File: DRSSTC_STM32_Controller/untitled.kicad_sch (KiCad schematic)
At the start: 46 parts, among them J4 Screw_Terminal_01x02, U3 LF15_TO252, U4 TPS54560BDDA, U7 LV2842XLVDDCR

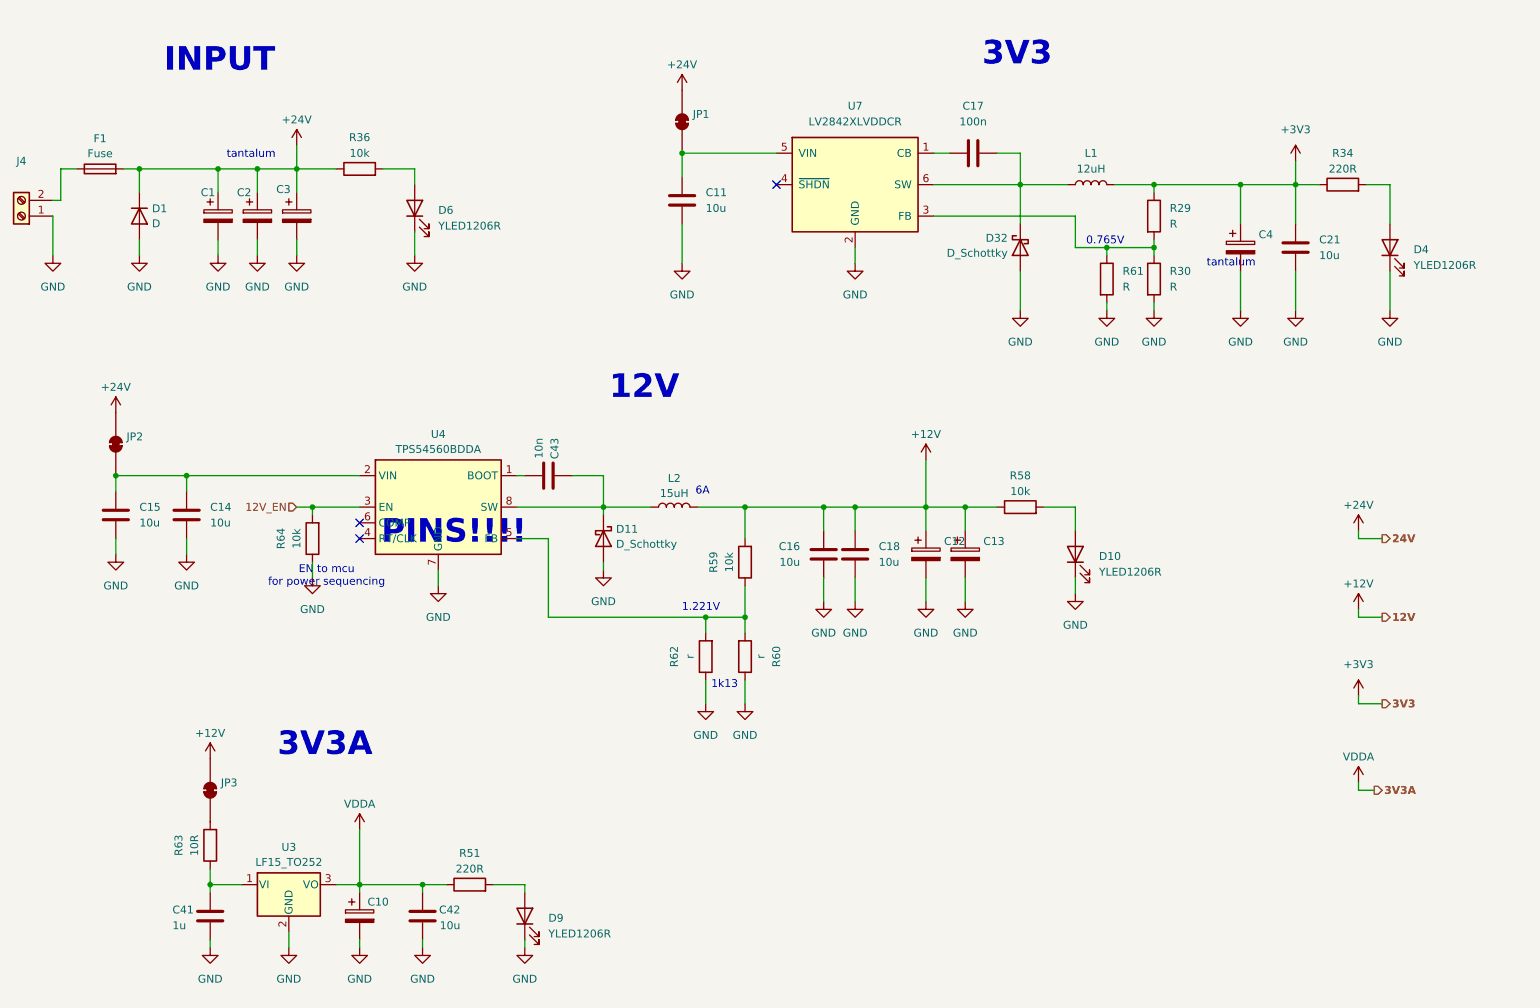
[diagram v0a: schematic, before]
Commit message: update conroller schematics
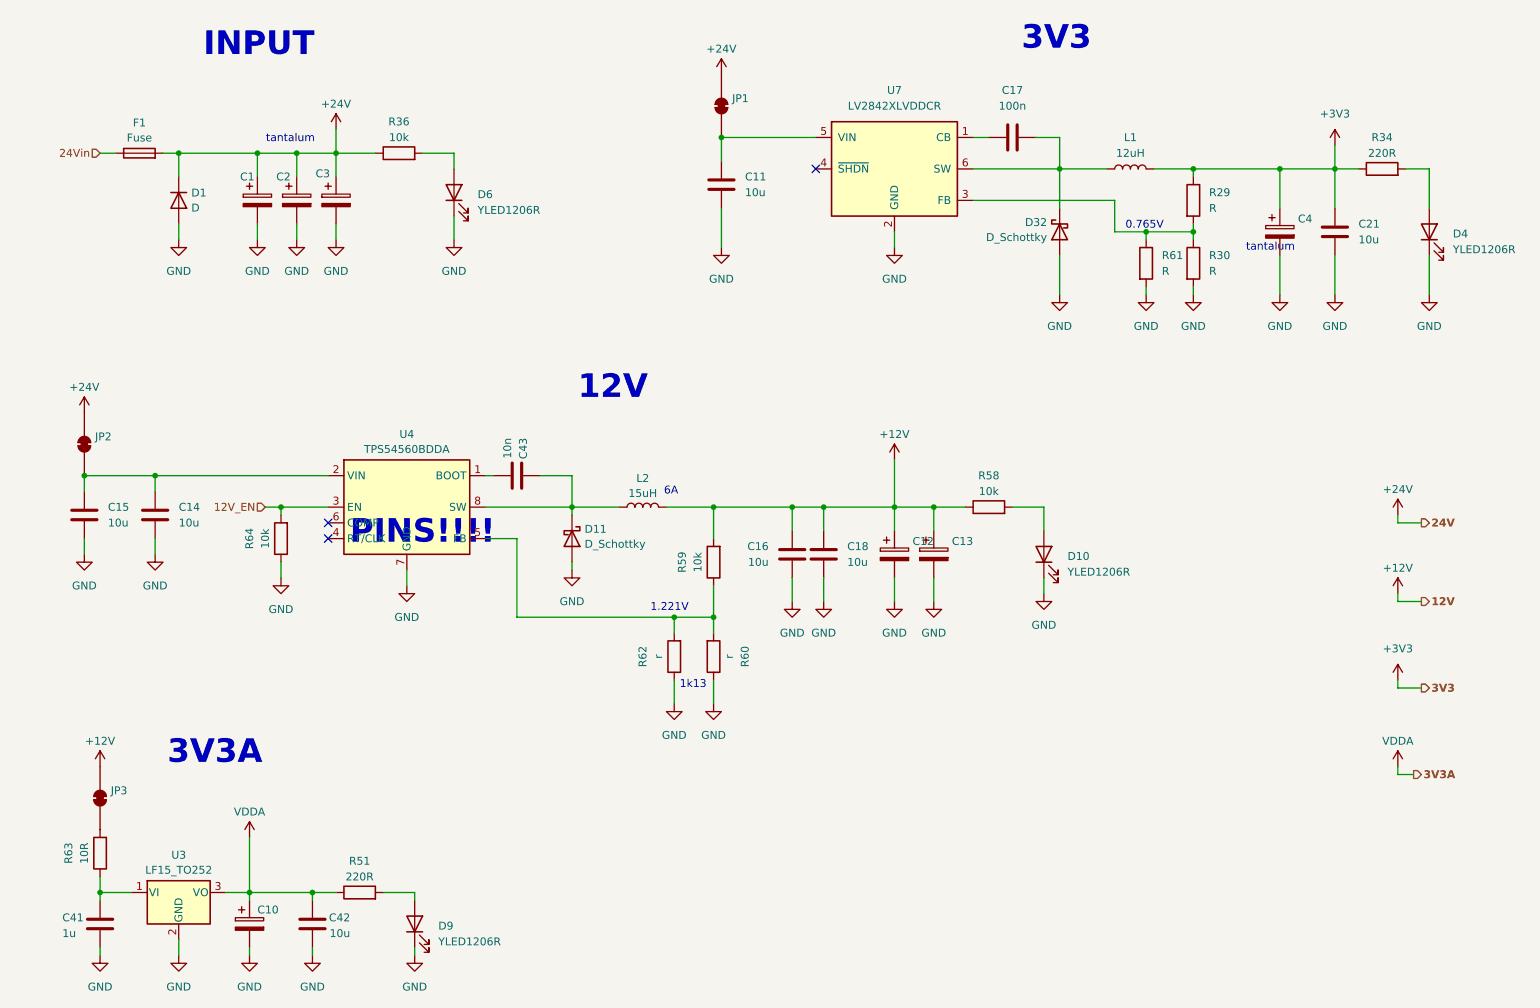
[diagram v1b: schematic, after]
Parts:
- removed J4: Screw_Terminal_01x02, TerminalBlock_Altech:Altech_AK100_1x02_P5.00mm, symbol Connector:Screw_Terminal_01x02
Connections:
- net 24Vin: now reaches F1.1
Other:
- note removed: "EN to mcu for power sequencing"
- moved on the sheet: C1, C10, C11, C12, C13, C14, C15, C16, C17, C18, C2, C21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
